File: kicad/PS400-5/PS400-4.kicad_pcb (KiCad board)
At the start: 2 copper layers, 13.5 x 13.1 mm, 28 parts, among them J1 +BAT, J2 +GM, J3 -BAT, J4 -GM, Q1 RUM002N05, Q2 Q_NPN_BEC, Q3 RUM002N05, T1 B82801A150, U2 PIC10F206-IOT

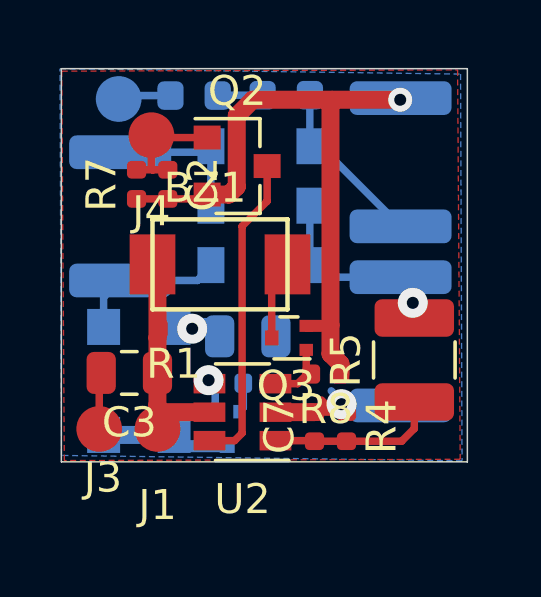
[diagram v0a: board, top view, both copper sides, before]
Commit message: изменено:      kicad/PS400-5/PS400-4.kicad_pcb 	изменено:      kicad/PS400-5/PS400-4.kicad_pcb-bak 	изменено:      kicad/PS400-5/fp-info-cache
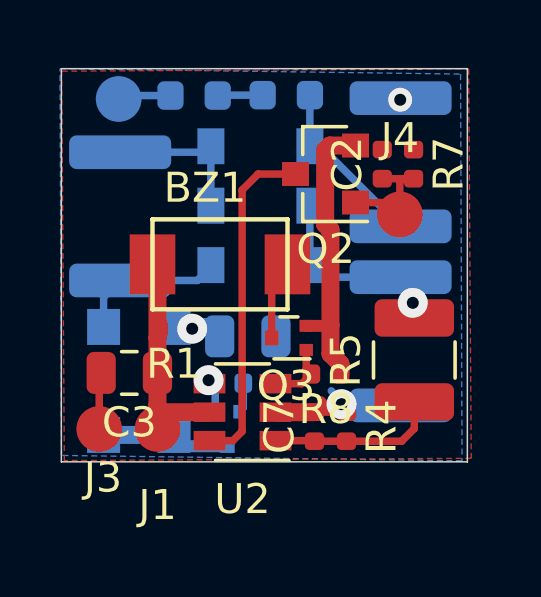
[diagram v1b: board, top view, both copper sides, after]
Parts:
- moved R7 9.26 mm to (43.5, 45.8), turned to 270 degrees
- moved J4 8.69 mm to (43.1, 47.5), turned to 180 degrees
- moved C2 7.18 mm to (42.5, 45.8), turned to 90 degrees
- moved Q2 2.96 mm to (40.6, 46.1), turned to 180 degrees
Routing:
- net GND: track 30.7 -> 18.6 mm
- net Net-(Q2-Pad3): track 10.4 -> 11.3 mm
